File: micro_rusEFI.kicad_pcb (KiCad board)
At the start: 4 copper layers, 80.6 x 93.7 mm, 180 parts, among them J1 USB_B_Micro, J19 Conn_01x06, J2 Conn_02x05_Odd_Even, J7 TC2030, SW1 SW_Push, SW2 SW_Push, SW3 SW_Push, SW4 SW_Push, U1 STM32F427VGT6, U2 LMR14020, U3 molex_48pin_MRE, U35 MCP6004, U36 MCP6004, U4 TJA1051T-3, U46 MCP6004, U5 LM1117-3.3, U6 TJA1051T-3, U8 MCP6004, X1 8MHz 20pF, Y2 32768 Hz

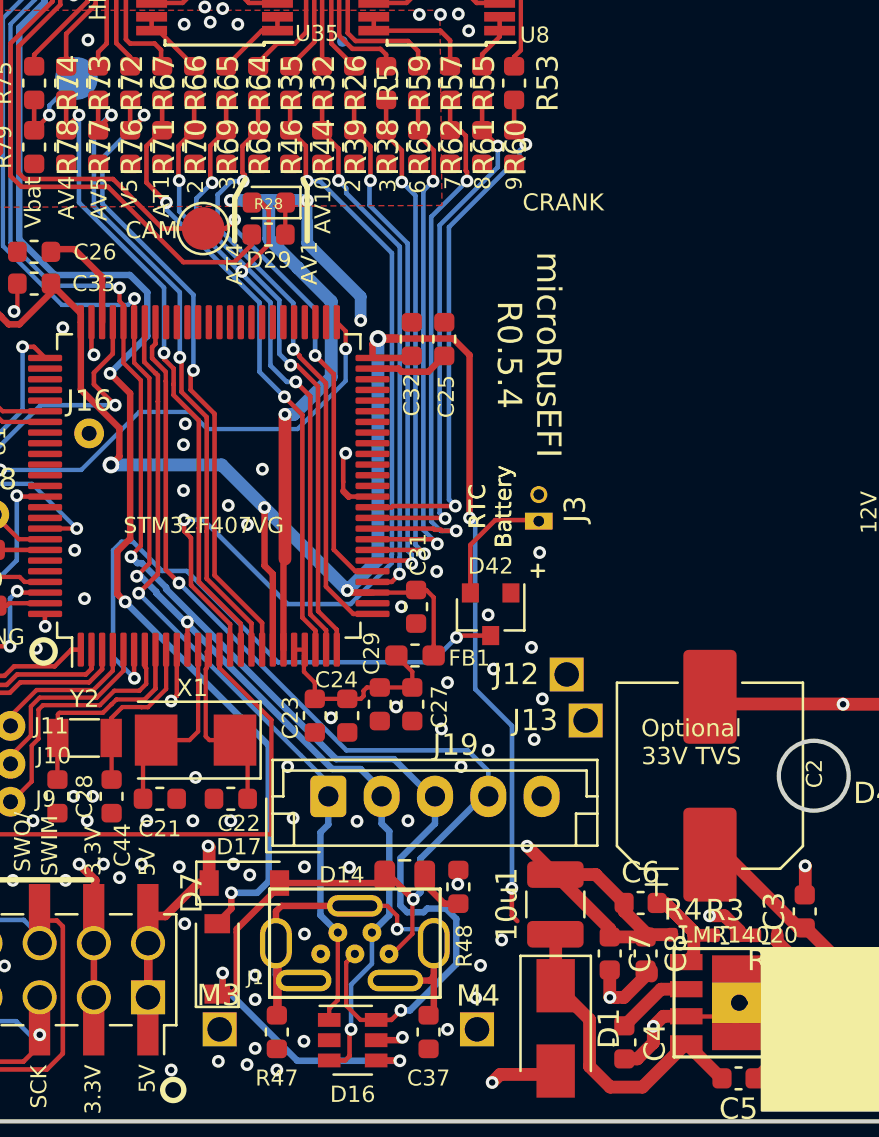
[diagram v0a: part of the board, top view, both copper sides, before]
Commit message: Fixing tags
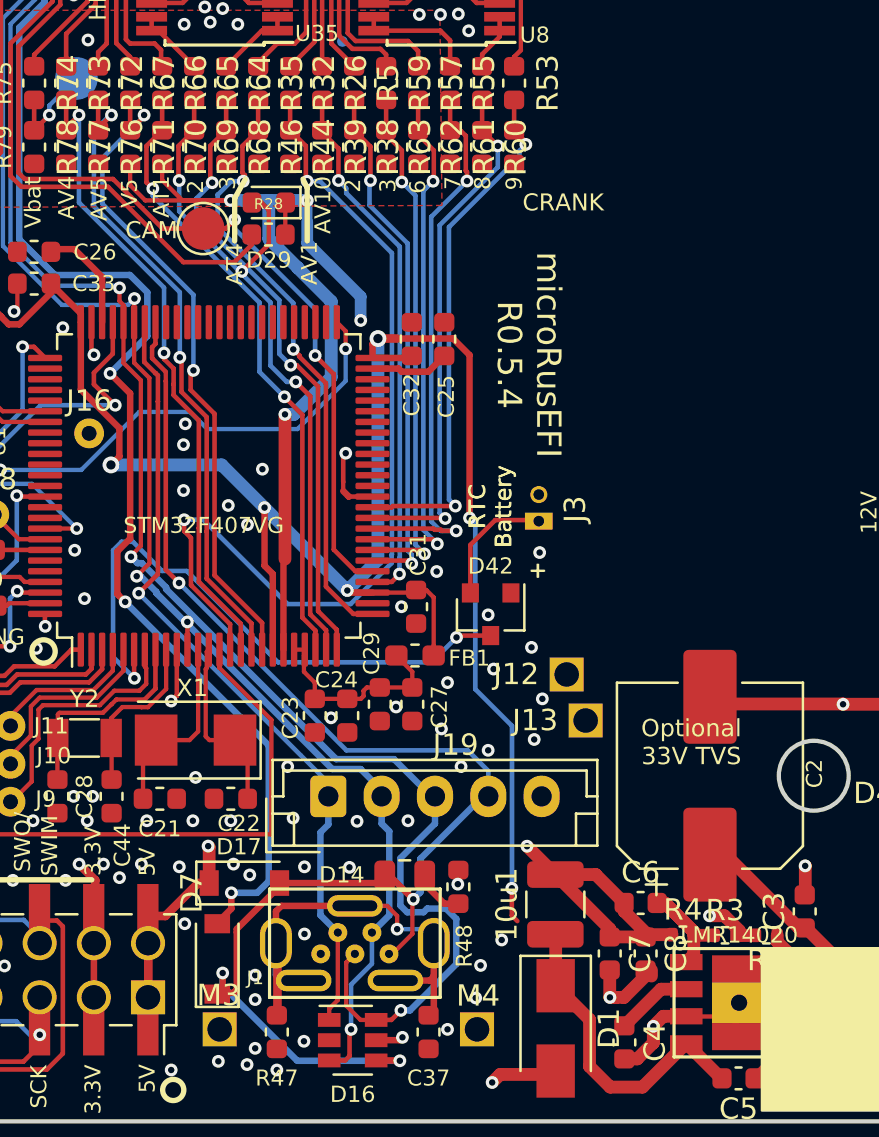
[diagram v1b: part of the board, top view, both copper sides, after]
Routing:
- net /ADC/AGND: track 27.0 -> 37.3 mm
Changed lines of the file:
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@@
   (via (at 49.6824 57.4802) (size 0.6) (drill 0.3) (layers "F.Cu" "B.Cu") (net 1))
   (via (at 55 87.2) (size 0.6) (drill 0.3) (layers "F.Cu" "B.Cu") (net 1))
-  (via (at 79.216592 110.522348) (size 0.6) (drill 0.3) (layers "F.Cu" "B.Cu") (net 1))
+  (via (at 78.950449 110.517255) (size 0.6) (drill 0.3) (layers "F.Cu" "B.Cu") (net 1))
   (via (at 44.293286 44.657115) (size 0.6) (drill 0.3) (layers "F.Cu" "B.Cu") (net 1))
   (via (at 83.82 96.52) (size 0.6) (drill 0.3) (layers "F.Cu" "B.Cu") (free) (net 1))
@@
   (segment (start 52.697212 73.403792) (end 52.697212 71.965293) (width 0.2159) (layer "B.Cu") (net 70))
   (segment (start 56.977001 77.683581) (end 52.697212 73.403792) (width 0.2159) (layer "B.Cu") (net 70))
-  (segment (start 51.16464 72.064636) (end 52.100004 73) (width 0.2159) (layer "F.Cu") (net 71))
+  (segment (start 51.461883 72.3465) (end 51.16464 72.049257) (width 0.2159) (layer "F.Cu") (net 71))
   (segment (start 58.472361 92.455841) (end 58.472361 82.945397) (width 0.2159) (layer "F.Cu") (net 71))
   (segment (start 51.9 68.1875) (end 51.9 69.6125) (width 0.2159) (layer "F.Cu") (net 71))
-  (segment (start 51.16464 70.34786) (end 51.16464 72.064636) (width 0.2159) (layer "F.Cu") (net 71))
-  (segment (start 51.9 69.6125) (end 51.16464 70.34786) (width 0.2159) (layer "F.Cu") (net 71))
+  (segment (start 51.16464 72.049257) (end 51.16464 70.34786) (width 0.2159) (layer "F.Cu") (net 71))
   (segment (start 59.0868 93.9596) (end 59.0868 93.07028) (width 0.2159) (layer "F.Cu") (net 71))
   (segment (start 59.0868 93.07028) (end 58.472361 92.455841) (width 0.2159) (layer "F.Cu") (net 71))
+  (segment (start 51.16464 70.34786) (end 51.9 69.6125) (width 0.2159) (layer "F.Cu") (net 71))
   (segment (start 57.632561 82.105597) (end 58.472361 82.945397) (width 0.2159) (layer "F.Cu") (net 71))
   (via (at 57.632561 82.105597) (size 0.6) (drill 0.3) (layers "F.Cu" "B.Cu") (net 71))
-  (via (at 52.100004 73) (size 0.6) (drill 0.3) (layers "F.Cu" "B.Cu") (net 71))
-  (segment (start 52.100004 73.327454) (end 52.100004 73) (width 0.2159) (layer "B.Cu") (net 71))
-  (segment (start 56.462648 80.935684) (end 56.462648 77.690098) (width 0.2159) (layer "B.Cu") (net 71))
-  (segment (start 56.462648 77.690098) (end 52.100004 73.327454) (width 0.2159) (layer "B.Cu") (net 71))
-  (segment (start 57.632561 82.105597) (end 56.462648 80.935684) (width 0.2159) (layer "B.Cu") (net 71))
+  (via (at 51.461883 72.3465) (size 0.6) (drill 0.3) (layers "F.Cu" "B.Cu") (net 71))
+  (segment (start 51.461883 72.689333) (end 56.462648 77.690098) (width 0.2159) (layer "B.Cu") (net 71))
+  (segment (start 51.461883 72.3465) (end 51.461883 72.689333) (width 0.2159) (layer "B.Cu") (net 71))
+  (segment (start 56.462648 77.690098) (end 56.462648 80.935684) (width 0.2159) (layer "B.Cu") (net 71))
+  (segment (start 56.462648 80.935684) (end 57.632561 82.105597) (width 0.2159) (layer "B.Cu") (net 71))
   (segment (start 54.8875 69.6125) (end 54.156957 70.343043) (width 0.2159) (layer "F.Cu") (net 72))
   (segment (start 59.20898 81.62066) (end 58.214436 80.626116) (width 0.2159) (layer "F.Cu") (net 72))
@@
   (segment (start 45.9 66.6125) (end 45.9 66.075) (width 0.2159) (layer "F.Cu") (net 118))
   (segment (start 45.917229 53.920871) (end 45.96168 53.87642) (width 0.2159) (layer "F.Cu") (net 118))
+  (segment (start 52.849135 72.9) (end 55.1 72.9) (width 0.2032) (layer "F.Cu") (net 119))
+  (segment (start 51.9 71.1875) (end 51.9 71.950865) (width 0.2032) (layer "F.Cu") (net 119))
   (segment (start 57.5868 93.9596) (end 57.5868 89.9576) (width 0.3048) (layer "F.Cu") (net 119))
+  (segment (start 51.111196 72.9) (end 55.1 72.9) (width 0.2032) (layer "F.Cu") (net 119))
   (segment (start 66.9 71.1875) (end 66.9 71.37068) (width 0.2159) (layer "F.Cu") (net 119))
+  (segment (start 50.4 72.188804) (end 51.111196 72.9) (width 0.2032) (layer "F.Cu") (net 119))
+  (segment (start 50.4 71.1875) (end 50.4 72.188804) (width 0.2032) (layer "F.Cu") (net 119))
   (segment (start 57.658 82.931) (end 57.658 89.7128) (width 0.6) (layer "F.Cu") (net 119))
+  (segment (start 51.9 71.950865) (end 52.849135 72.9) (width 0.2032) (layer "F.Cu") (net 119))
   (via (at 58.7 72.9) (size 0.6) (drill 0.3) (layers "F.Cu" "B.Cu") (net 119))
   (via (at 55.1 72.9) (size 0.6) (drill 0.3) (layers "F.Cu" "B.Cu") (net 119))
